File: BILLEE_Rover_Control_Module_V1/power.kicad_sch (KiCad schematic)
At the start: 96 parts, among them CN2 XT60PW-M, U10 TPS1HA08BQPWPRQ1, U11 LT8612EUDE#TRPBF, U14 +12V_COMMS_PWR, U2 TPS1HA08BQPWPRQ1, U23 TPS1HA08BQPWPRQ1, U24 LT8612EUDE#TRPBF, U25 +12V_AUX_PWR, U5 TPS1HA08BQPWPRQ1, U6 INA780BIDEKR, U7 LT8612EUDE#TRPBF, U8 LT8612EUDE#TRPBF, U9 +20V_JETSON_PWR

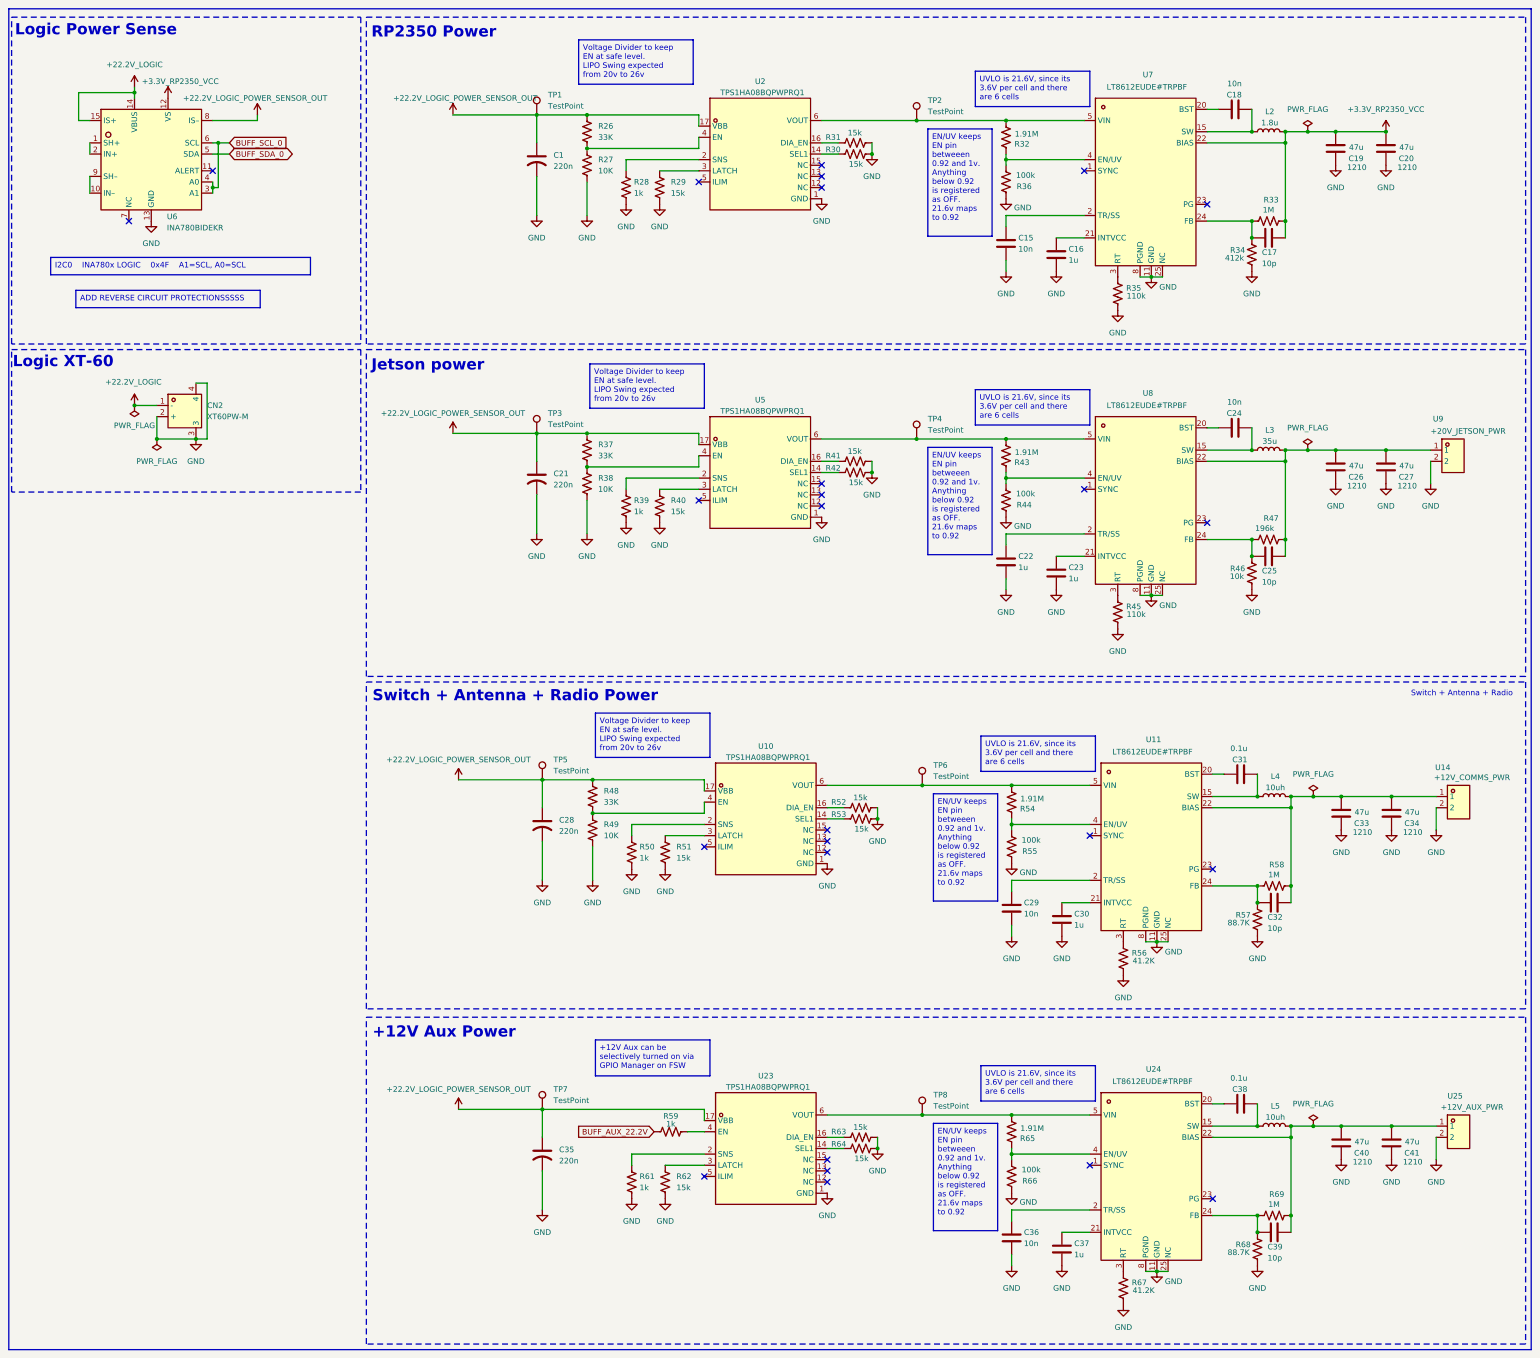
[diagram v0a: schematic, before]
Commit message: WIP Checkpoint
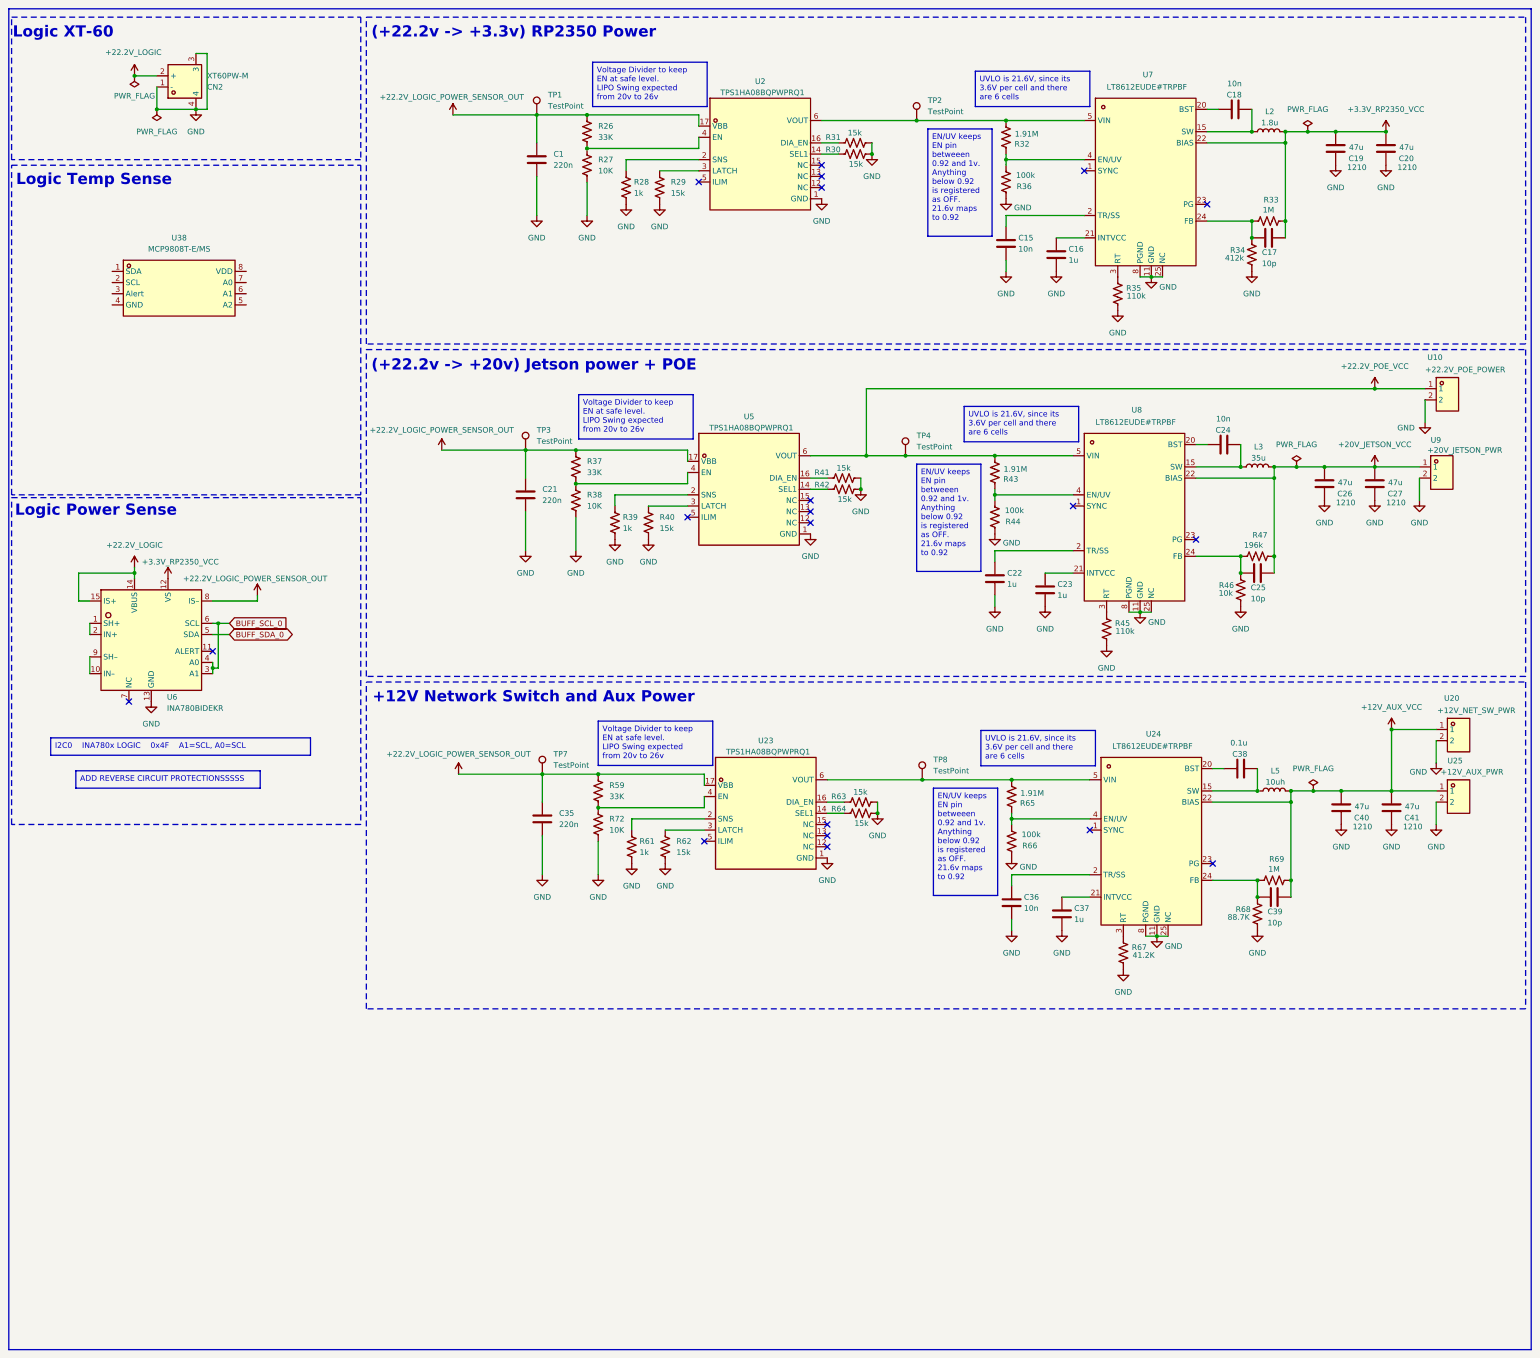
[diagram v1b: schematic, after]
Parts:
- removed C28: 220n, symbol Device:C_US
- removed C29: 10n, symbol Device:C
- removed C30: 1u, symbol Device:C
- removed C31: 0.1u, symbol Device:C
- removed C32: 10p, symbol Device:C
- removed C33, C34: 47u, symbol Device:C
- removed L4: 10uh, symbol Device:L
- removed R48: 33K, symbol Device:R_US
- removed R49: 10K, symbol Device:R_US
- removed R50: 1k, symbol Device:R_US
- removed R51, R52, R53: 15k, symbol Device:R_US
- removed R54: 1.91M, symbol Device:R_US
- removed R55: 100k, symbol Device:R_US
- removed R56: 41.2K, symbol Device:R_US
- removed R57: 88.7K, symbol Device:R_US
- removed R58: 1M, symbol Device:R_US
- removed TP5, TP6: TestPoint, Connector_Pin:Pin_D1.0mm_L10.0mm, symbol Connector:TestPoint
- removed U10: TPS1HA08BQPWPRQ1, PDB_LCSC:HTSSOP-16_L5.0-W4.4-P0.65-LS6.4-BL-EP, symbol PDB_LCSC_Libs:TPS1HA08BQPWPRQ1
- removed U11: LT8612EUDE#TRPBF, PDB_LCSC:QFN-28_L6.0-W3.0-P0.50-BL-EP, symbol PDB_LCSC_Libs:LT8612EUDE#TRPBF
- removed U14: +12V_COMMS_PWR, PDB_LCSC:CONN-TH_P5.00_KF301-5.0-2P, symbol PDB_LCSC_Libs:KF301-5.0-2P
- added R72: 10K, symbol Device:R_US
- added U10: +22.2V_POE_POWER, PDB_LCSC:CONN-TH_P5.00_KF301-5.0-2P, symbol PDB_LCSC_Libs:KF301-5.0-2P
- added U20: +12V_NET_SW_PWR, PDB_LCSC:CONN-TH_P5.00_KF301-5.0-2P, symbol PDB_LCSC_Libs:KF301-5.0-2P
- added U38: MCP9808T-E/MS, PDB_LCSC:MSOP-8_L3.0-W3.0-P0.65-LS4.9-BL, symbol PDB_LCSC_Libs:MCP9808T-E_MS
- C1, C21, C35: symbol Device:C_US -> Device:C
- R59: value 1k -> 33K
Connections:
- net BUFF_AUX_22.2V is gone; now on net +22.2V_LOGIC_POWER_SENSOR_OUT: R59.1
- net +22.2V_LOGIC: now also CN2.2 (+); no longer CN2.1 (-)
- net GND: now also CN2.1 (-), R72.2, U10.2, U20.2; no longer CN2.2 (+)
- net +12V_AUX_VCC: now reaches C39.1, C40.1, C41.1, L5.2, R69.1, U24.22 (BIAS), U25.1
- net +12V_AUX_VCC: now also U20.1
- net +20V_JETSON_VCC: now reaches C25.1, C26.1, C27.1, L3.2, R47.1, U8.22 (BIAS), U9.1
- net +22.2V_POE_VCC: now reaches R43.2, TP4.1, U5.6 (VOUT), U8.5 (VIN)
- net +22.2V_POE_VCC: now also U10.1
- net at R59.2, U23.4 (EN): now also R72.1
- no-connect marks 26 -> 20
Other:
- note added: "(+22.2v -> +20v) Jetson power + POE"
- note added: "(+22.2v -> +3.3v) RP2350 Power"
- note added: "+12V Network Switch and Aux Power"
- note added: "Logic Temp Sense"
- note removed: "+12V Aux Power"
- note removed: "Jetson power"
- note removed: "RP2350 Power"
- note removed: "Switch + Antenna + Radio"
- note removed: "Switch + Antenna + Radio Power"
- moved on the sheet: C21, C22, C23, C24, C25, C26, C27, C35, C36, C37, C38, C39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

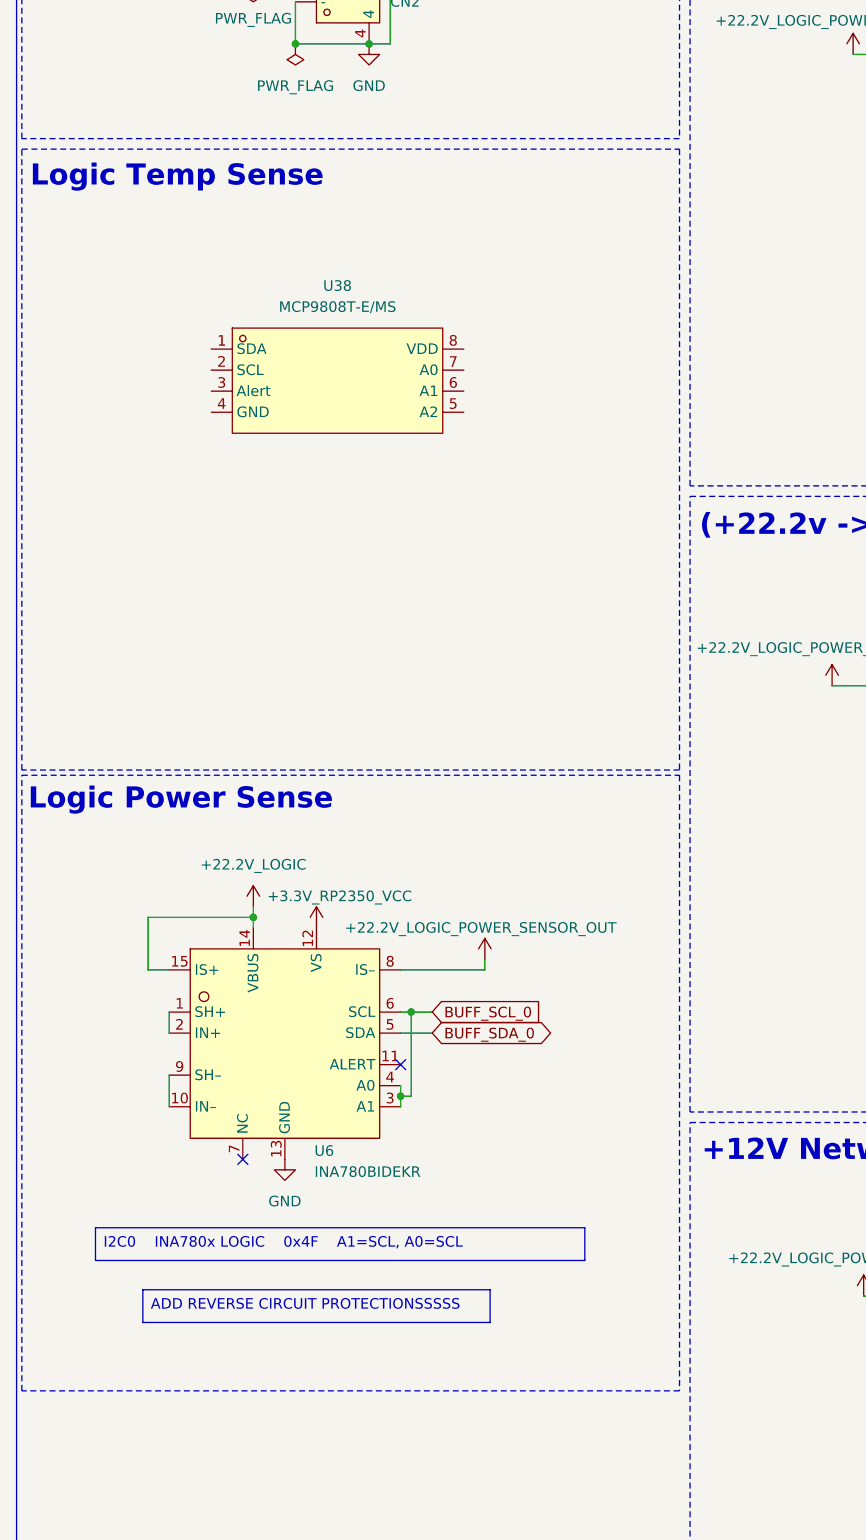
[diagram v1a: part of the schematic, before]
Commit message: Goodies
Updated all schematics
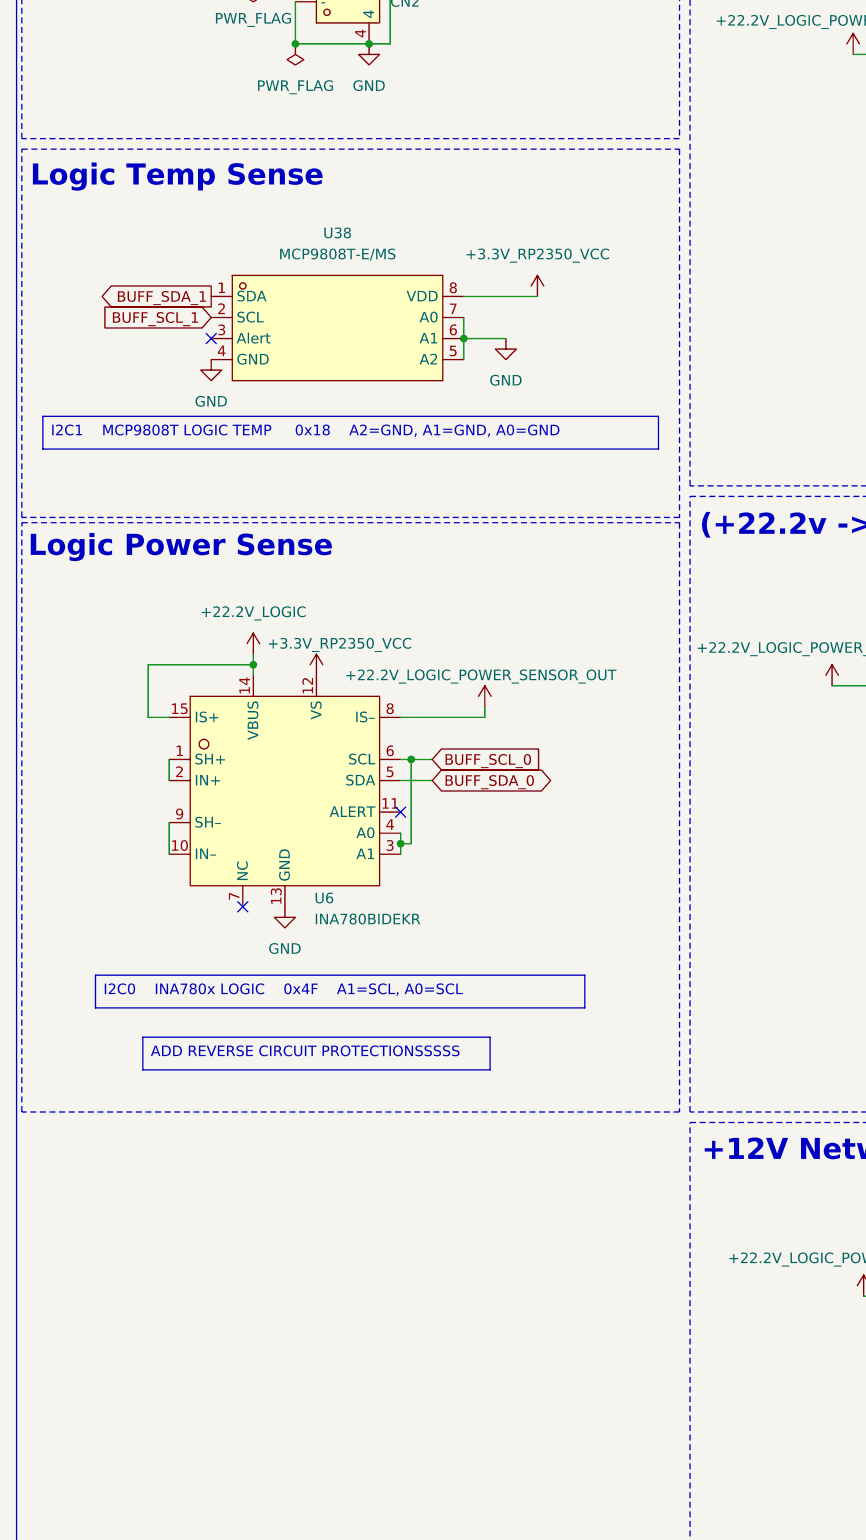
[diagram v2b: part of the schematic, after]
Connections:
- net +3.3V_RP2350_VCC: now also U38.8 (VDD)
- net GND: now also U38.4 (GND), U38.5 (A2), U38.6 (A1), U38.7 (A0)
- net BUFF_SDA_1: now reaches U38.1 (SDA)
- net BUFF_SCL_1: now reaches U38.2 (SCL)
- no-connect marks 20 -> 21
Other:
- company: (none) -> Bronco STAR
- title: (none) -> BILLEE_RCM
- moved on the sheet: U38, U6
